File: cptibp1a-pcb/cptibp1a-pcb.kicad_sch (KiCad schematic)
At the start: 24 parts, among them J1 10118194-0001LF, J2 PAD+, J3 PAD-, Q1 2N7002, Q2 AO3413, U1 NCP360SNT, U2 APX809S-31SA, U3 BQ21040, U4 APX810S-44SA, U5 NCP380HSN05

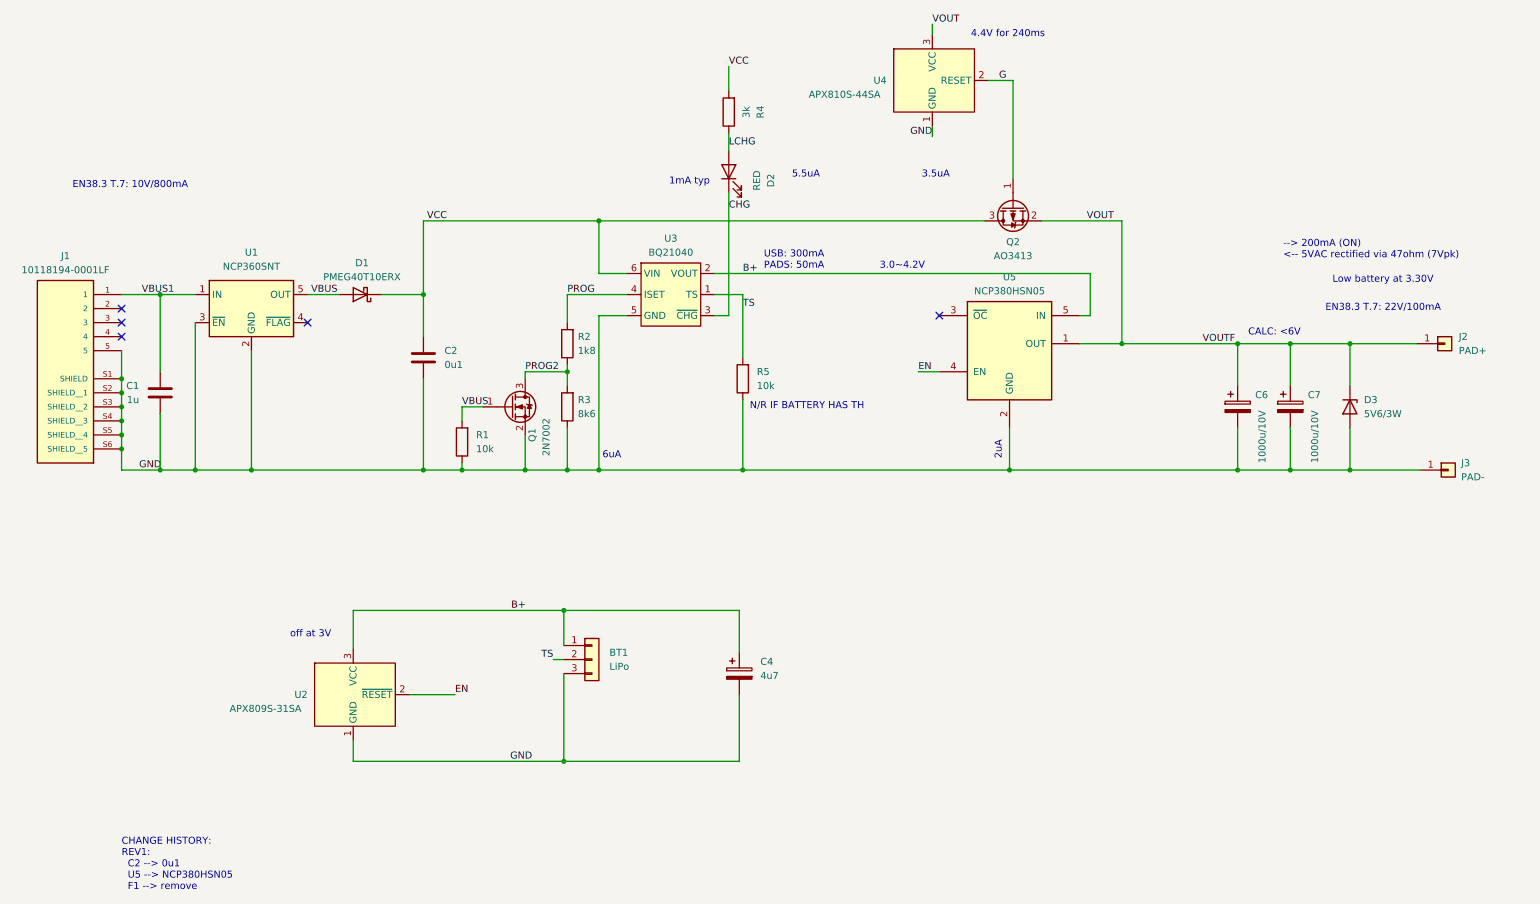
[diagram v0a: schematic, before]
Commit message: rev1
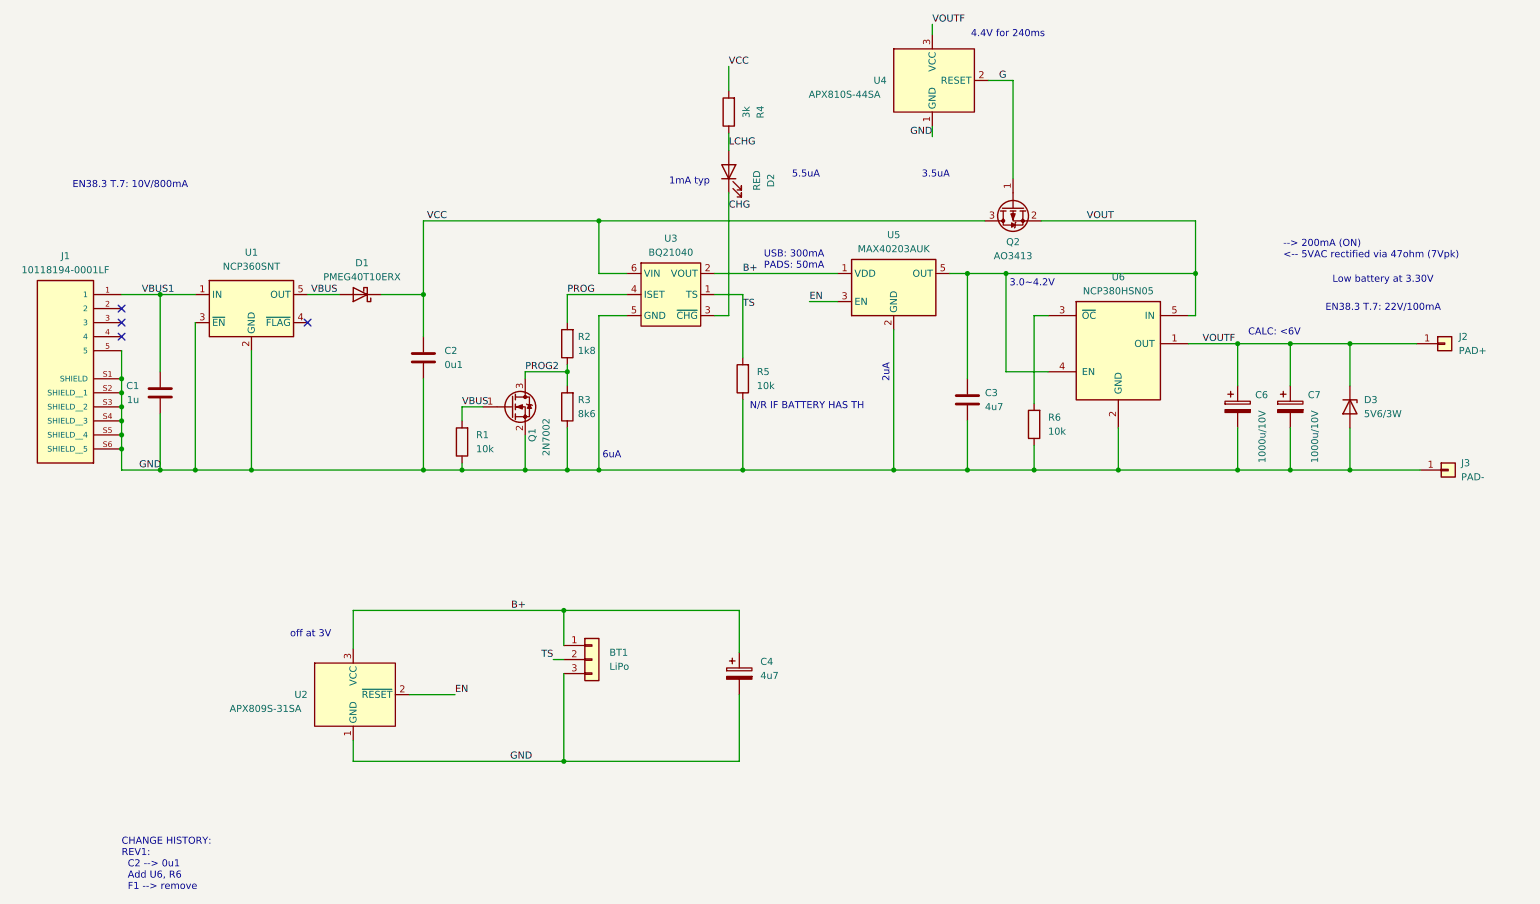
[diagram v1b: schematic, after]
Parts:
- added C3: 4u7, Capacitor_SMD:C_0805_2012Metric, symbol Device:C
- added R6: 10k, Resistor_SMD:R_0805_2012Metric, symbol Device:R
- added U5: MAX40203AUK, george:SOT-23-5_TI_DBV5, symbol Analog_Switch:MAX40200AUK
- renumbered U5 to U6
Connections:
- net B+: now also U5.1 (VDD); no longer U6.5 (IN)
- net EN: now also U5.3 (EN); no longer U6.4 (EN)
- net GND: now also C3.2, R6.1, U5.2 (GND)
- net VOUT: now also U6.4 (EN), U6.5 (IN), C3.1, U5.5 (OUT); no longer C6.1, C7.1, D3.1 (K), J2.1 (Pin_1), U4.3 (VCC), U6.1 (OUT)
- net at U6.3 (~{OC}): now also R6.2
- new net VOUTF: C6.1, C7.1, D3.1 (K), J2.1 (Pin_1), U4.3 (VCC), U6.1 (OUT)
- no-connect marks 5 -> 4
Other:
- note added: "CHANGE HISTORY: REV1: C2 --> 0u1 Add U6, R6 F1 --> remove"
- note removed: "CHANGE HISTORY: REV1: C2 --> 0u1 U5 --> NCP380HSN05 F1 --> remove"
- moved on the sheet: U6
